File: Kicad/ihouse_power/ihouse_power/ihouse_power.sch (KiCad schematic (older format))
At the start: 23 parts, among them J10 Conn_02x07_Odd_Even, J11 Conn_01x06, J12 Conn_01x06, J14 Optic, J15 Hum1, J16 Hum2, J17 Hum3, J18 Temp, J19 I2C, J21 RS232, J22 Nextion, J5 Conn_01x16, J6 Conn_01x06, J7 Conn_02x07_Odd_Even, J8 Conn_01x16, J9 Conn_01x06, M3 ev1527receiver_module, U12 MAX232

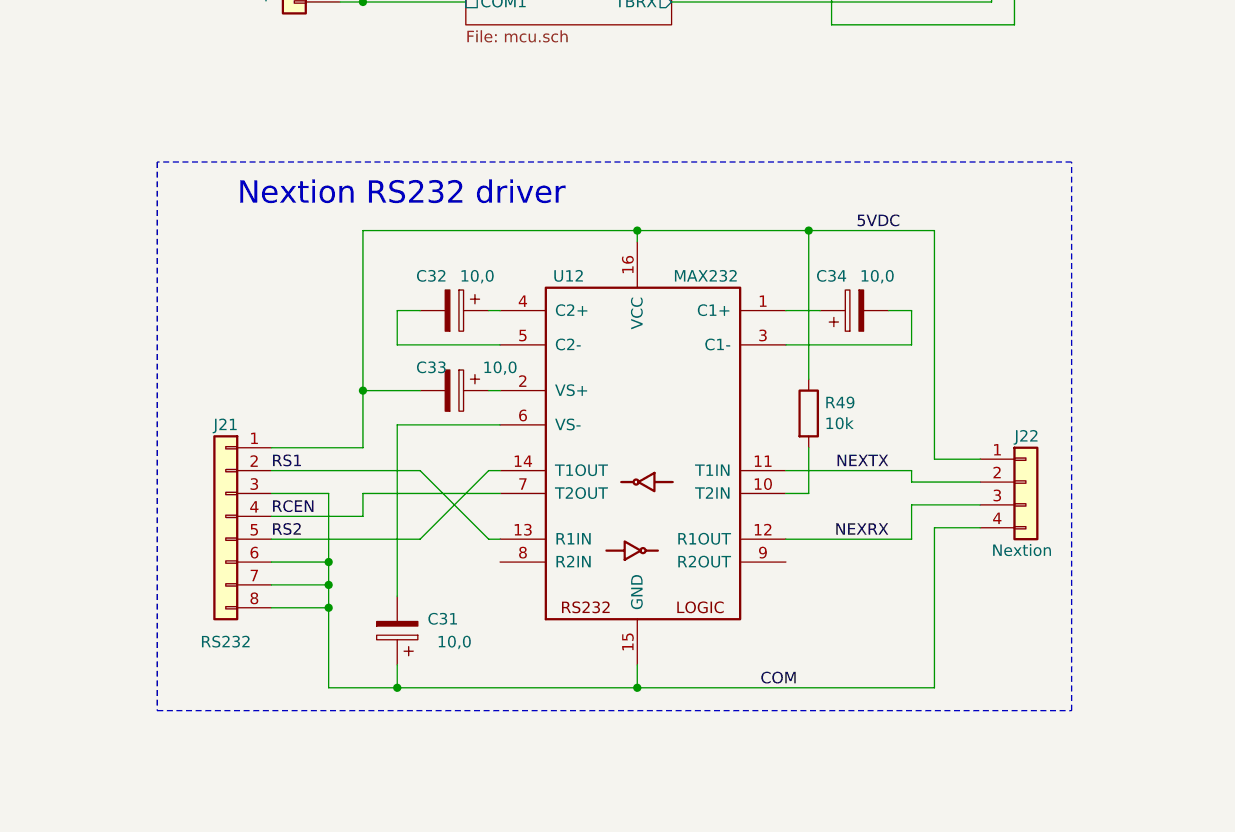
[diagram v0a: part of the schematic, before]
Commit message: tarpinis komitas
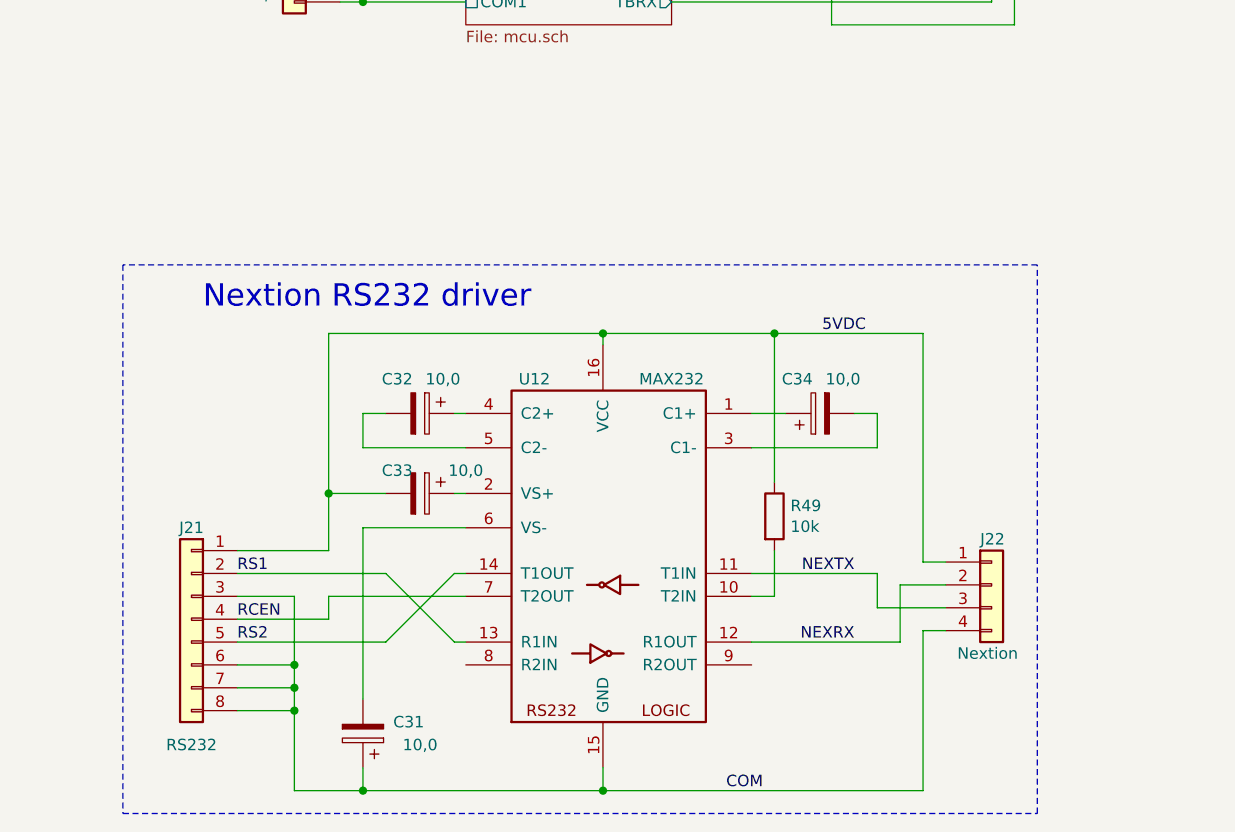
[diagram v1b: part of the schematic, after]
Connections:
- net NEXRX: now also J22.2 (Pin_2); no longer J22.3 (Pin_3)
- net NEXTX: now also J22.3 (Pin_3); no longer J22.2 (Pin_2)
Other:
- moved on the sheet: C31, C32, C33, C34, J21, J22, R49, U12
